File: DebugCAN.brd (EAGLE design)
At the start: 56 x 63 mm, 58 parts, among them J1 8P8C-LED, J2 XT60PW-M, J3 MA04-1, J4 10118192-0001LF, J5 8P8C-LED, J6 8P8C-LED, J7 8P8C-LED, U1 STM32F302C, U2 NCV7351D1E, U3 SI8621AB-B-IS, U4 AP2127N-3.3TRG1, U5 78L05F, U6 TLP291, X1 CSTCE8M00G55

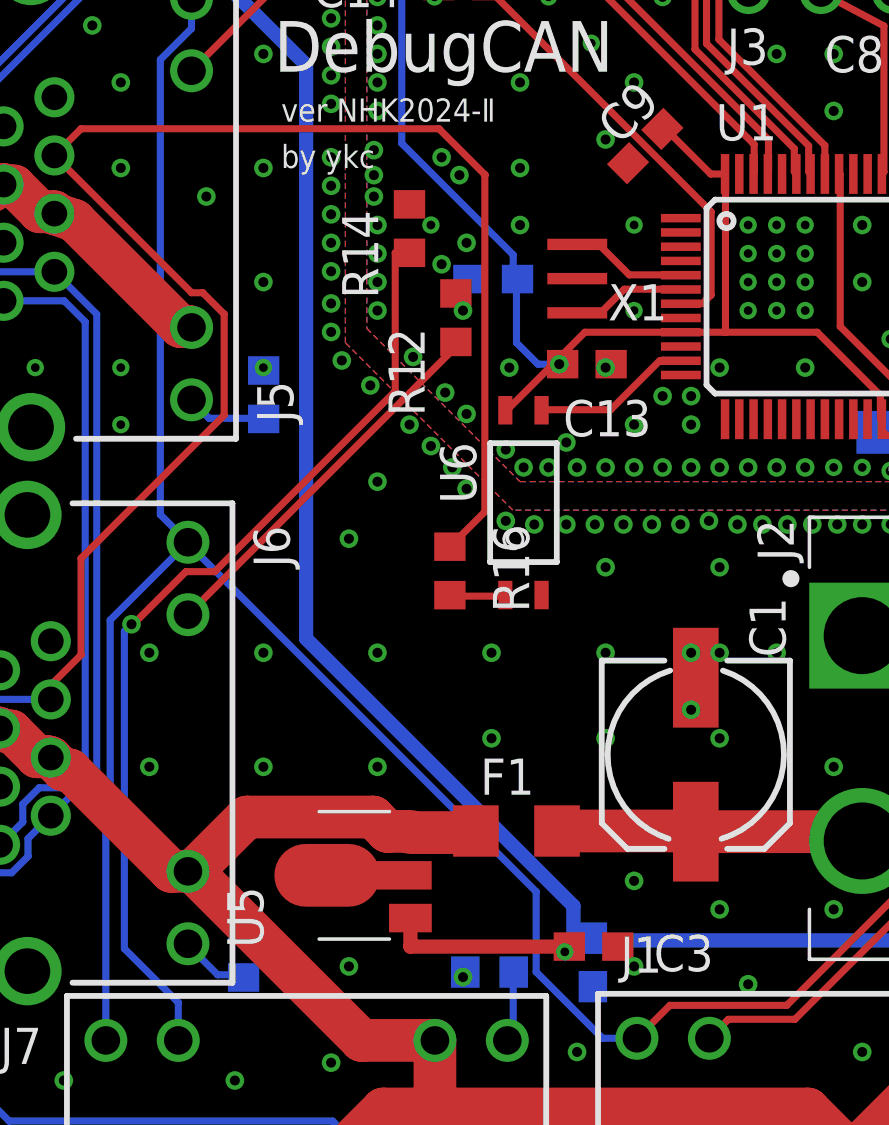
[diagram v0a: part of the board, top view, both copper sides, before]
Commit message: update
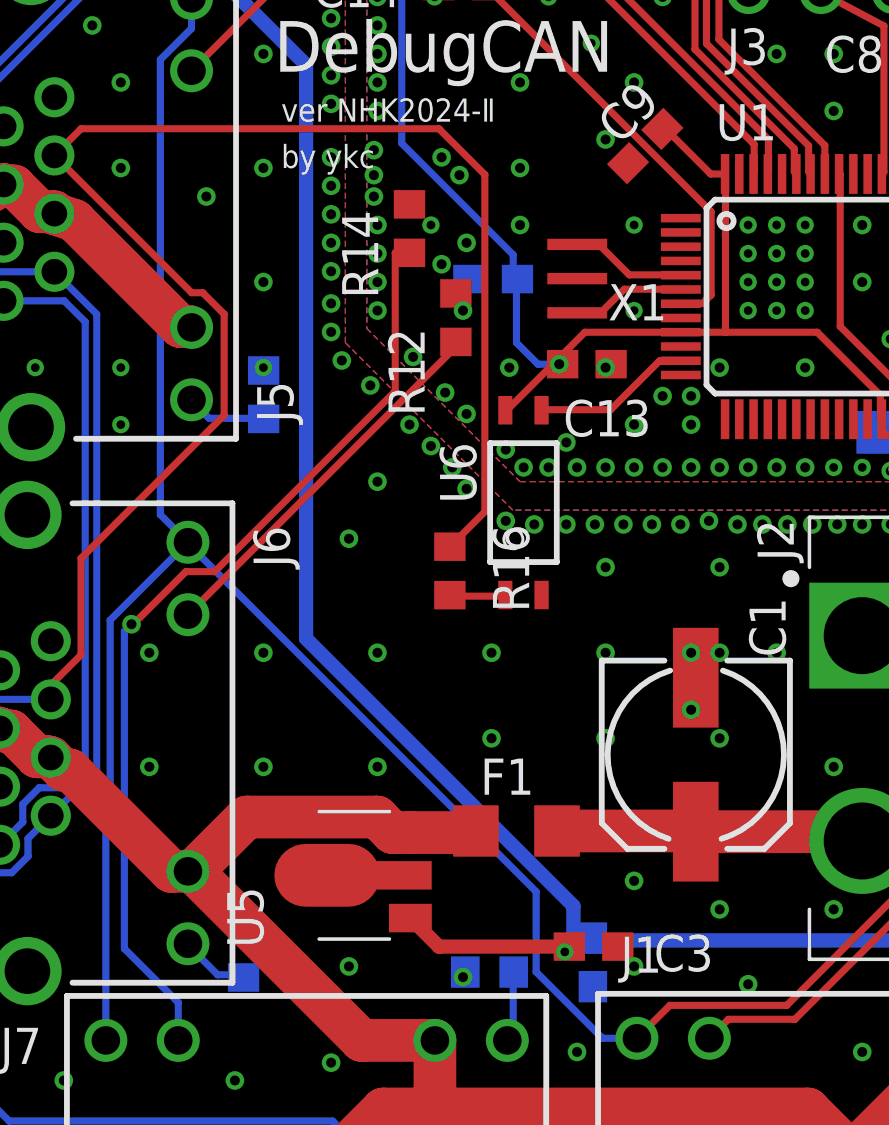
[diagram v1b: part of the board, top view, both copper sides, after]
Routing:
- net +5V_ISO: track 89.3 -> 88.7 mm
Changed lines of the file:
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@@
 <wire x1="10.4624" y1="25.3512" x2="10.545" y2="25.325" width="1.5" layer="1"/>
 <wire x1="8.8528" y1="26.2566" x2="8.765" y2="26.345" width="1.5" layer="1"/>
-<wire x1="22.3512" y1="22.7356" x2="23.156" y2="22.7356" width="1.5" layer="1"/>
-<wire x1="22.3512" y1="22.7356" x2="21.8482" y2="23.2386" width="1.5" layer="1"/>
 <wire x1="2.771" y1="39.9656" x2="7.419434375" y2="44.614034375" width="1.5" layer="1"/>
 <wire x1="2.771" y1="30.7104" x2="2.771" y2="39.9656" width="1.5" layer="1"/>
@@
 <wire x1="24.015" y1="15.405" x2="24.015" y2="13.015" width="1.5" layer="1"/>
 <wire x1="24.015" y1="13.015" x2="24" y2="13" width="1.5" layer="1"/>
-<wire x1="17.41678125" y1="23.2386" x2="15.51318125" y2="21.335" width="1.5" layer="1"/>
-<wire x1="21.8482" y1="23.2386" x2="17.41678125" y2="23.2386" width="1.5" layer="1"/>
+<wire x1="15.51318125" y1="21.335" x2="17.41678125" y2="23.2386" width="1.5" layer="1"/>
 <wire x1="10.545" y1="25.325" x2="10.9786" y2="24.8914" width="1.5" layer="1"/>
 <wire x1="10.9786" y1="24.8914" x2="11.21039375" y2="24.8914" width="1.5" layer="1"/>
@@
 <wire x1="23.156" y1="22.694" x2="25.397" y2="22.694" width="1.5" layer="1"/>
 <wire x1="25.397" y1="22.694" x2="25.453" y2="22.75" width="1.5" layer="1"/>
-<wire x1="23.156" y1="22.7356" x2="23.156" y2="22.694" width="0" layer="19" extent="1-1"/>
+<wire x1="17.41678125" y1="23.2386" x2="21.9864" y2="23.2386" width="1.5" layer="1"/>
+<wire x1="22.531" y1="22.694" x2="23.156" y2="22.694" width="1.5" layer="1"/>
+<wire x1="22.531" y1="22.694" x2="21.9864" y2="23.2386" width="1.5" layer="1"/>
 </signal>
 <signal name="+5V_ISO" class="1">
@@
 <wire x1="19.5164" y1="60.5612" x2="19.52" y2="60.505" width="0.5" layer="16"/>
 <wire x1="15.6936" y1="58.1468" x2="16.47" y2="58.055" width="0.5" layer="16"/>
-<wire x1="23.156" y1="18.695" x2="28.73" y2="18.695" width="0.5" layer="1"/>
-<wire x1="23.156" y1="18.695" x2="23.156" y2="19.696" width="0.5" layer="1"/>
+<wire x1="24.156" y1="18.695" x2="28.73" y2="18.695" width="0.5" layer="1"/>
+<wire x1="24.156" y1="18.696" x2="23.156" y2="19.696" width="0.5" layer="1"/>
+<wire x1="24.156" y1="18.696" x2="24.156" y2="18.695" width="0.5" layer="1"/>
 <wire x1="28.9728" y1="18.9128" x2="29.4758" y2="18.9128" width="0.5" layer="16"/>
 <wire x1="28.5704" y1="18.5104" x2="28.9728" y2="18.9128" width="0.5" layer="16"/>
@@
 <wire x1="33.25" y1="3.5" x2="34.6086" y2="4.8586" width="0.25" layer="1"/>
 <wire x1="34.6086" y1="4.8586" x2="34.6086" y2="9.2965125" width="0.25" layer="1"/>
-<wire x1="25.778" y1="45.7547" x2="25.76635" y2="45.76635" width="0.25" layer="1"/>
 <contactref element="U$1" pad="P$1"/>
 <wire x1="25.76635" y1="45.76635" x2="24.1561" y2="47.3766" width="0.25" layer="1"/>
@@
 <signal name="DCIN" class="2">
 <contactref element="C1" pad="+"/>
-<wire x1="33.134" y1="22.694" x2="33.165" y2="22.725" width="1.5" layer="1"/>
-<wire x1="33.19" y1="22.75" x2="33.165" y2="22.725" width="1.5" layer="1"/>
 <contactref element="F1" pad="2"/>
 <contactref element="J2" pad="2"/>
-<wire x1="28.297" y1="22.75" x2="33.19" y2="22.75" width="1.5" layer="1"/>
+<wire x1="33.19" y1="22.75" x2="28.297" y2="22.75" width="1.5" layer="1"/>
 <wire x1="33.165" y1="22.725" x2="38.675" y2="22.725" width="1.5" layer="1"/>
 <wire x1="38.675" y1="22.725" x2="39" y2="22.4" width="1.5" layer="1"/>
+<wire x1="33.165" y1="22.725" x2="33.19" y2="22.75" width="1.5" layer="1"/>
 </signal>
 </signals>
